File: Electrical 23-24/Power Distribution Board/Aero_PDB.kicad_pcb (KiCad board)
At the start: 2 copper layers, 72.6 x 89.9 mm, 28 parts, among them J1 Conn_01x04_Pin, J101 Gimbal Conn, J102 Pixhawk Servo Conn, J103 Pixawk Backup Power, J104 USB_OTG, J105 Servo to PDB Conn, J106 JST_XH_4, J107 DCJ200-10-A-XX-K_REVA, J108 JST_XH_4, J2 Conn_01x04_Pin, J3 RCIN, J4 RCIN, Q201 PNP, Q202 PNP

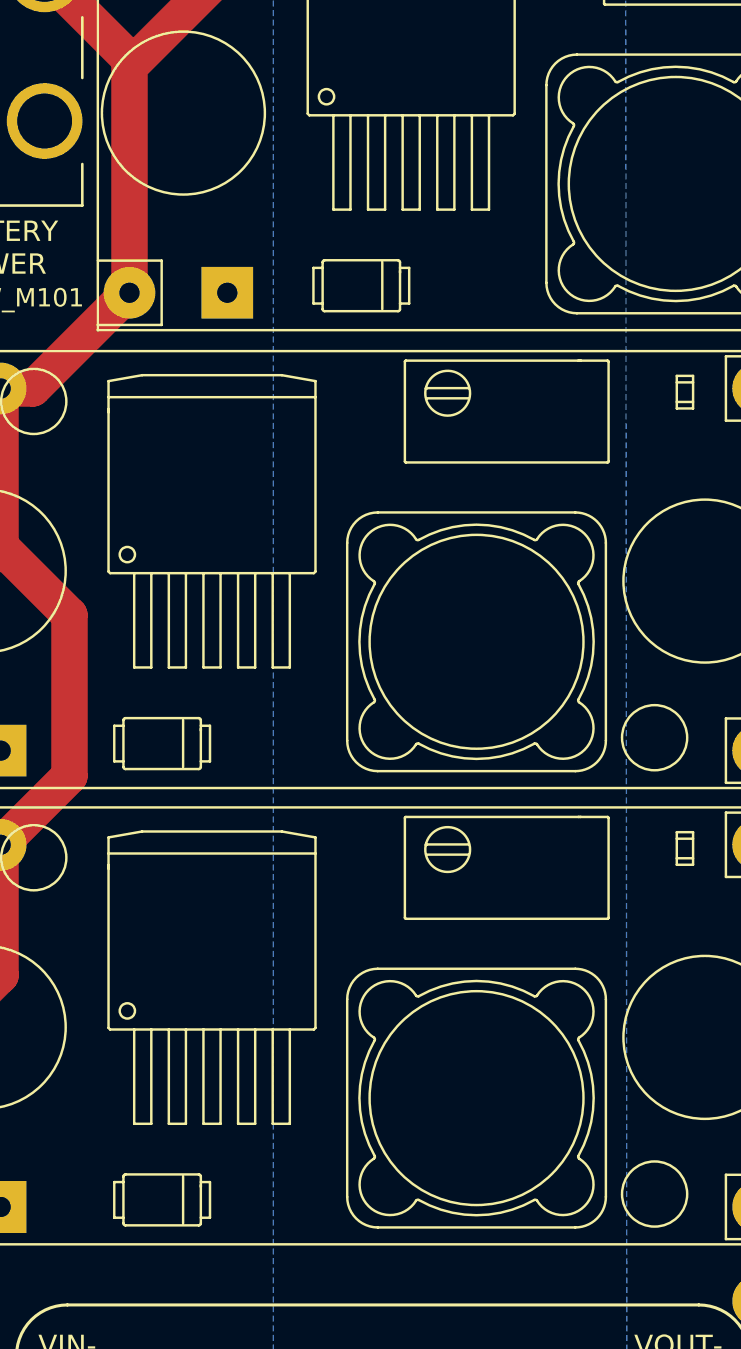
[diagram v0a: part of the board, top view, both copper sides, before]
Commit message: Fix a MAJOR issue that ANTHONY caused
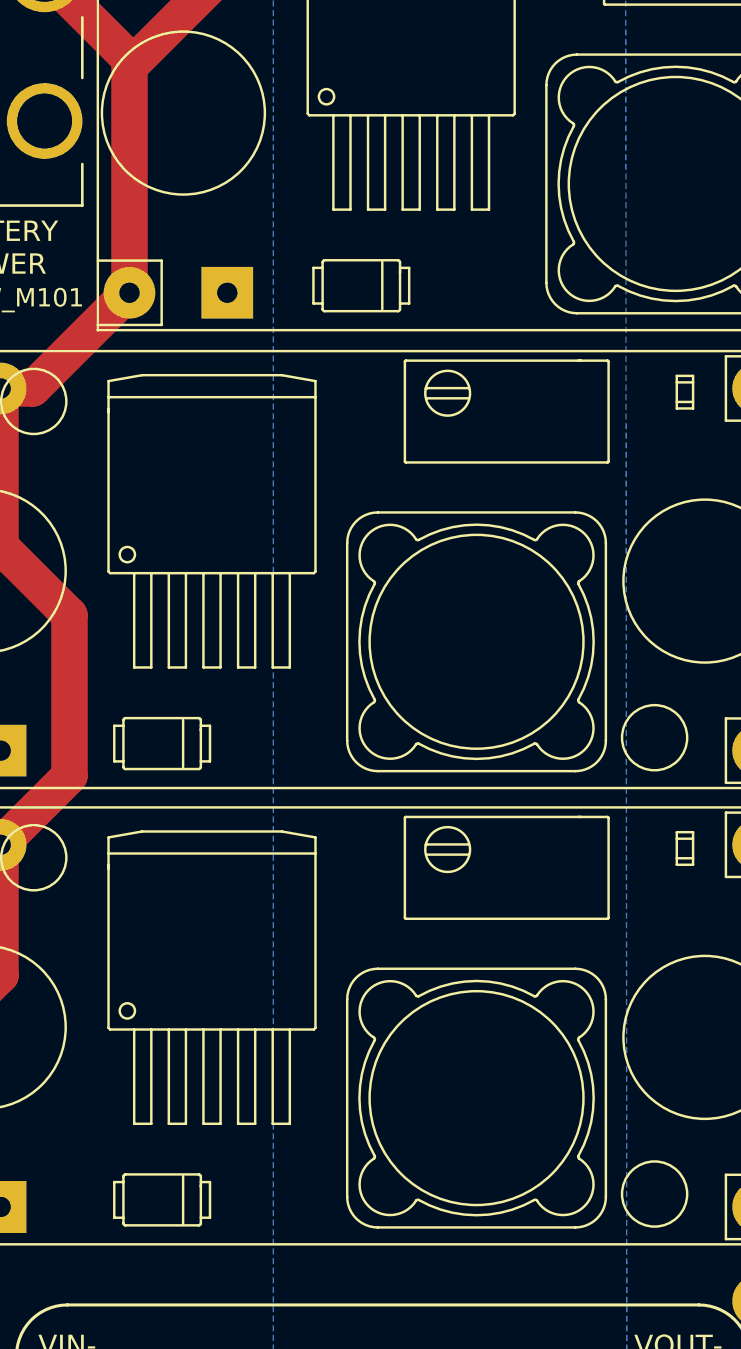
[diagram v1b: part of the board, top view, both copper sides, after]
